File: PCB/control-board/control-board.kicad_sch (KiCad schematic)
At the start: 8 parts, among them J1 OLED, J2 PROGRAM, SW1 SW_Push, SW2 SW_Push, SW3 SW_Push, SW4 SW_Push, U1 ATtiny84A-SS

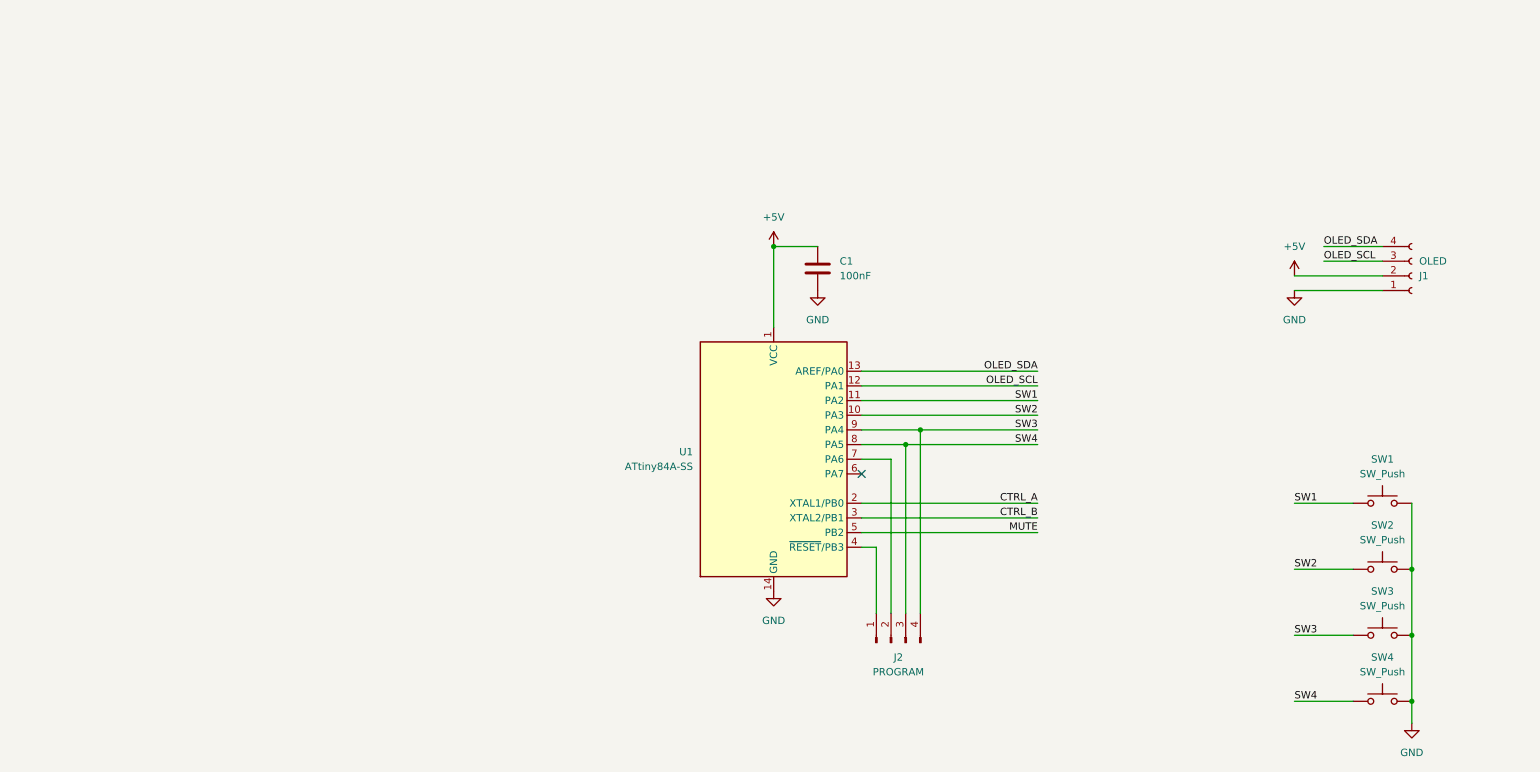
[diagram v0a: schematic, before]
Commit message: bom, readme, cad, pcb
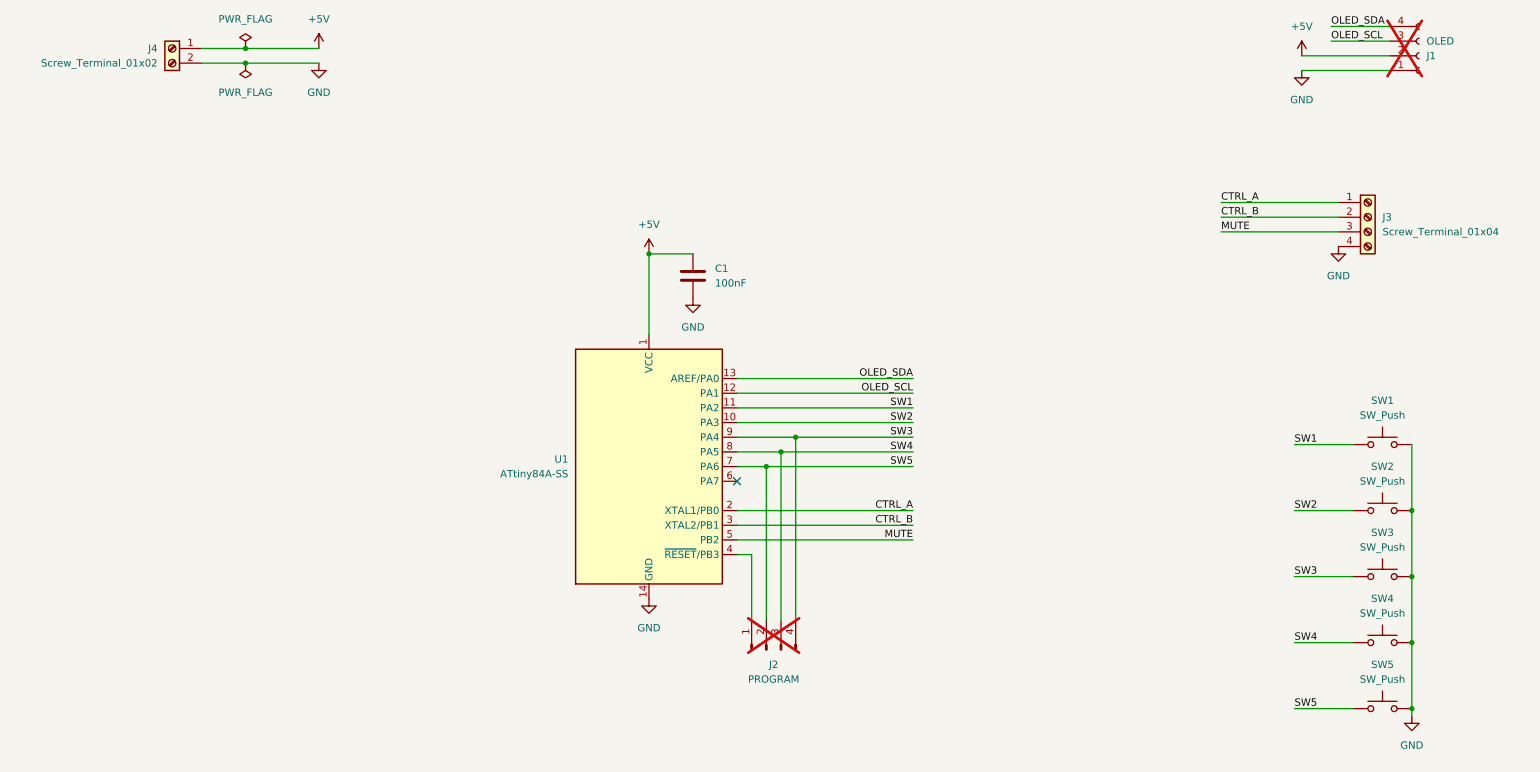
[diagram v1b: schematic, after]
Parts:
- added J3: Screw_Terminal_01x04, Connector_Phoenix_MSTB:PhoenixContact_MSTBA_2,5_4-G-5,08_1x04_P5.08mm_Horizontal, symbol Connector:Screw_Terminal_01x04
- added J4: Screw_Terminal_01x02, TerminalBlock_CUI:TerminalBlock_CUI_TB007-508-02_1x02_P5.08mm_Horizontal, symbol Connector:Screw_Terminal_01x02
- added SW5: SW_Push, Button_Switch_THT:SW_PUSH_6mm, symbol Switch:SW_Push
- J1: footprint (none) -> KiCad-SSD1306-0.91-OLED-4pin-128x32:SSD1306-0.91-OLED-4pin-128x32; now not fitted; now left out of the parts list
- J2: footprint (none) -> Connector_PinHeader_2.54mm:PinHeader_1x04_P2.54mm_Vertical; now not fitted; now left out of the parts list
- SW1, SW2, SW3, SW4: footprint (none) -> Button_Switch_THT:SW_PUSH_6mm; Mouser PN (none) -> 179-TS026655BK260LCR
- U1: Mouser PN (none) -> 556-ATTINY84A-SSFR
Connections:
- net +5V: now also J4.1 (Pin_1)
- net CTRL_A: now also J3.1 (Pin_1)
- net CTRL_B: now also J3.2 (Pin_2)
- net GND: now also J3.4 (Pin_4), J4.2 (Pin_2), SW5.2
- net MUTE: now also J3.3 (Pin_3)
- net SW5: now reaches J2.2 (Pin_2), U1.7 (PA6)
- net SW5: now also SW5.1
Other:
- moved on the sheet: C1, SW1, SW2, SW3, SW4, U1
